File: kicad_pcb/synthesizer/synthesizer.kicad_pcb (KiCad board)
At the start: 2 copper layers, 69.9 x 58.9 mm, 43 parts, among them J1 SCL_GND_SCA, J2 Fuente5V, J4 Fuente12V, J5 CONSMA006.062-G, Q1 BCW31_

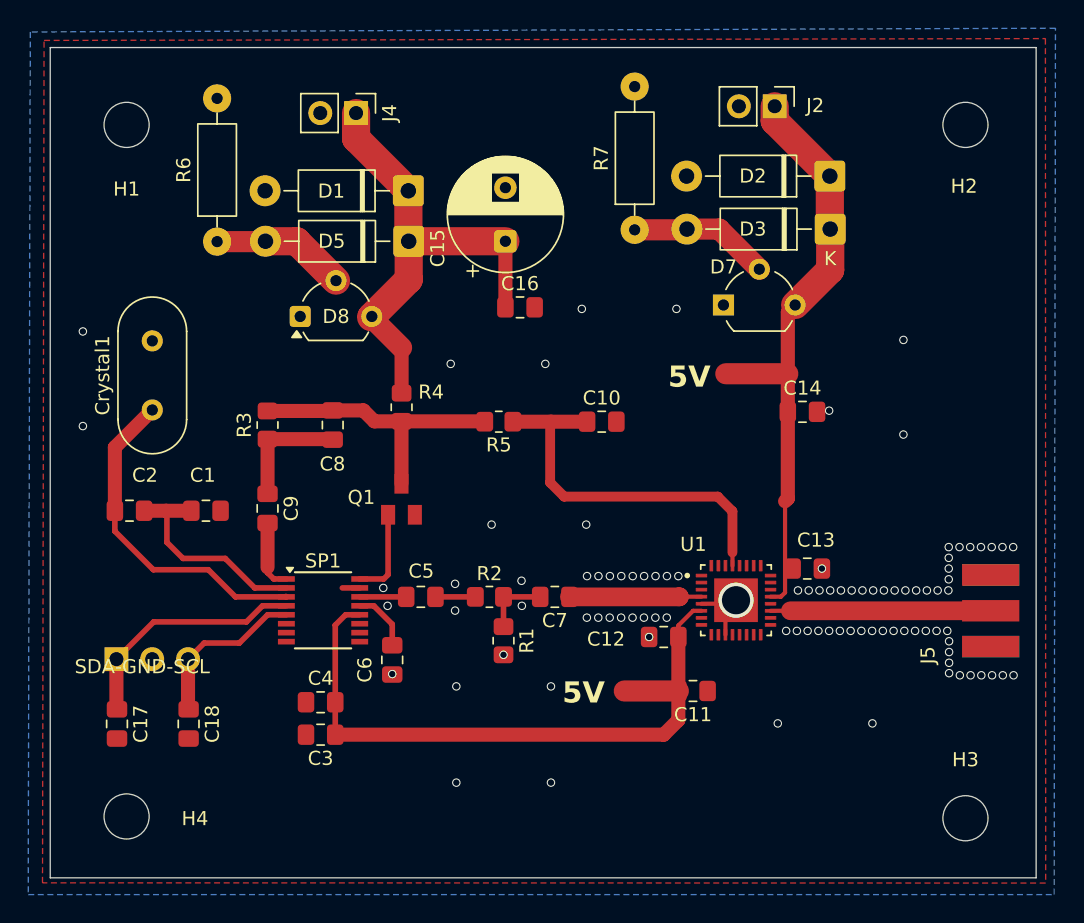
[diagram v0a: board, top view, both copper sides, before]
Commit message: Se modifica placa para nuevo integrado
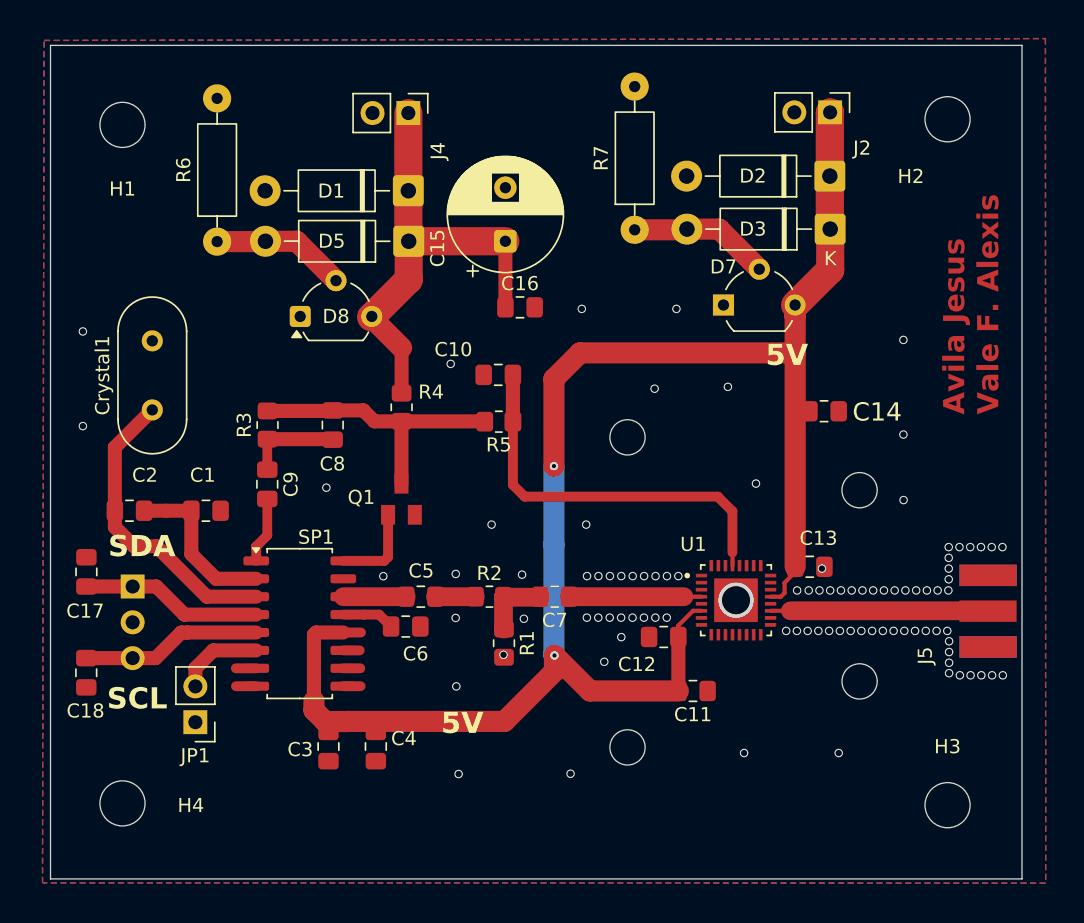
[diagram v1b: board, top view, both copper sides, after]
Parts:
- added H5: MountingHole, MountingHole:MountingHole_2.5mm, F.Cu at (202.5, 95.7)
- added H5: MountingHole, MountingHole:MountingHole_2.5mm, F.Cu at (186.0, 91.9)
- added H5: MountingHole, MountingHole:MountingHole_2.5mm, F.Cu at (202.5, 109.2)
- added H5: MountingHole, MountingHole:MountingHole_2.5mm, F.Cu at (186.0, 113.9)
- added JP1: Jumper_2_Bridged, Connector_PinHeader_2.54mm:PinHeader_1x02_P2.54mm_Vertical, F.Cu at (155.4, 112.1)
- J2: value Fuente5V -> 5V
- J4: value Fuente12V -> 12V
- SP1: footprint Package_SO:SSOP-16_3.9x4.9mm_P0.635mm -> Package_SO:SOP-16_4.4x10.4mm_P1.27mm
- moved C17 11.0 mm to (147.7, 101.5), turned to 90 degrees
- moved C18 8.12 mm to (147.6, 108.6)
- moved C10 8.05 mm to (176.9, 87.5), turned to 180 degrees
- moved J1 5.28 mm to (150.9, 102.5), turned to 180 degrees
- moved C4 5.02 mm to (168.2, 113.8), turned to -90 degrees
- moved J2 3.95 mm to (200.4, 68.9)
- moved J4 3.71 mm to (170.5, 68.9)
- moved C6 2.55 mm to (170.3, 105.3), turned to 180 degrees
- moved SP1 1.90 mm to (162.8, 105.1)
- moved C9 1.71 mm to (160.5, 95.2)
- moved H3 1.57 mm to (208.7, 118.0)
- moved C14 1.53 mm to (200.0, 90.1)
- moved H2 1.33 mm to (208.7, 69.3)
- moved C3 1.01 mm to (164.8, 113.8), turned to -90 degrees
- moved H4 0.97 mm to (150.2, 118.0)
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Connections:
- SP1 pad 6: unconnected-(SP1-Port_P3-Pad6) -> Net-(JP1-B)
- U1 pad 11: GND -> unconnected-(U1-GND-Pad11)
- U1 pad 5: GND -> unconnected-(U1-GND-Pad5)
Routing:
- net +5V: track 90.2 -> 119.4 mm, vias 0 -> 2
- net Net-(JP1-B): track 0.00 -> 6.12 mm
- net GND: track 6.55 -> 1.41 mm, vias 96 -> 95
- net Net-(J1-Pin_1): track 17.2 -> 12.9 mm
- net Net-(SP1-Crystal_Cap): track 15.4 -> 11.8 mm
- net Net-(SP1-Crystal): track 23.8 -> 21.5 mm
- net Net-(C8-Pad2): track 8.51 -> 6.81 mm
- net +12V: track 35.0 -> 33.5 mm
- net unconnected-(SP1-Port_P2-Pad7): track 0.00 -> 1.45 mm
- net unconnected-(SP1-Port_P1-Pad8): track 0.00 -> 1.44 mm
- net unconnected-(SP1-Port_P0-Pad9): track 0.00 -> 1.23 mm
- net unconnected-(SP1-Adress-Pad10): track 0.00 -> 1.21 mm
- net unconnected-(SP1-Ref/Comp-Pad11): track 0.00 -> 1.17 mm
- net Net-(C5-Pad2): track 3.30 -> 4.46 mm
- net Net-(J1-Pin_3): track 11.9 -> 12.8 mm
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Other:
- board size 69.9 x 58.9 mm -> 68.9 x 59.1 mm
- board text added: "Avila Jesus Vale F. Alexis"
- board text added: "GND"
- board text added: "SCL"
- board text added: "SDA"
- board text removed: "SDA-GND-SCL"
